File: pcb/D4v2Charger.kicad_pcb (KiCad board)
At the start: 2 copper layers, 21.6 x 20.6 mm, 16 parts, among them J1 Conn_01x02_Pin, U1 BQ25185DLHR

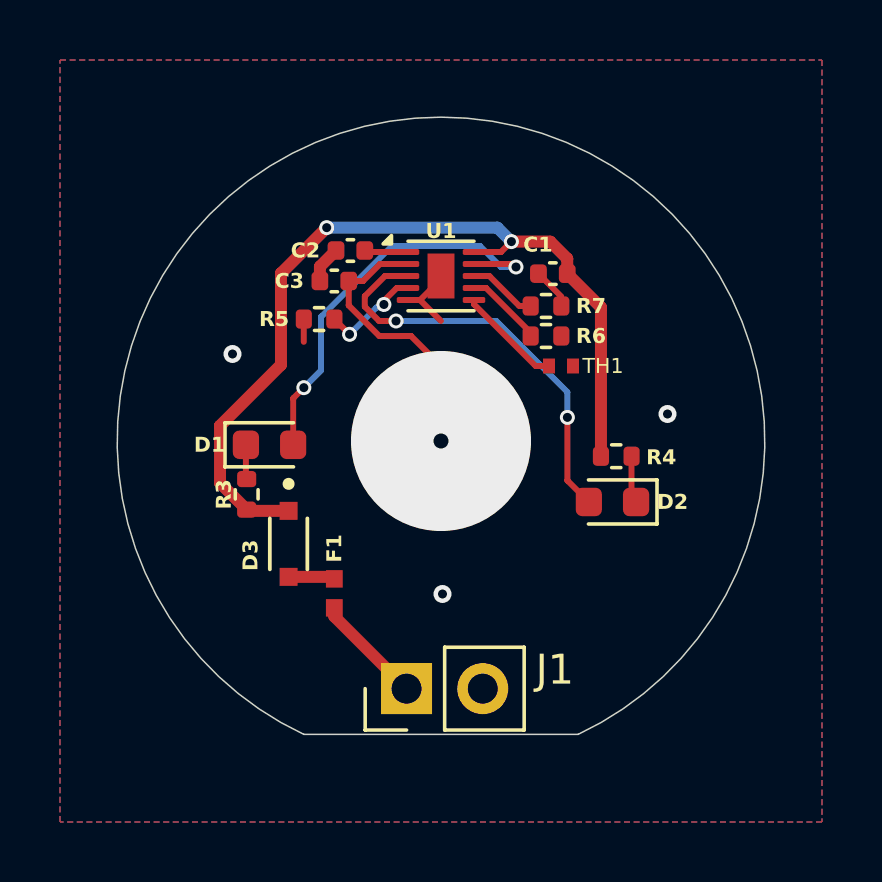
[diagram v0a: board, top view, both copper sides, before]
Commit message: update edge cuts
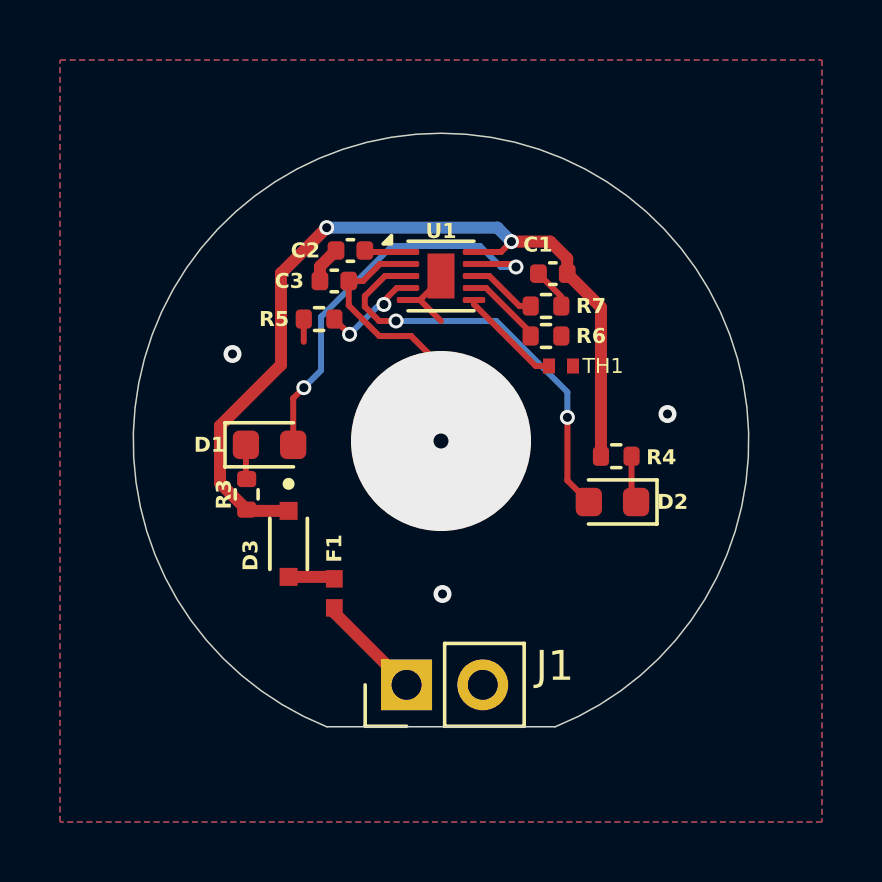
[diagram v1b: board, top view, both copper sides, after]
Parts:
- moved J1 0.13 mm to (170.3, 97.0)
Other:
- board size 21.6 x 20.6 mm -> 20.5 x 19.8 mm
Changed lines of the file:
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@@
 	(footprint "Connector_PinHeader_2.54mm:PinHeader_1x02_P2.54mm_Vertical"
 		(layer "F.Cu")
-		(at 170.302 97.155 90)
+		(at 170.302 97.028 90)
 		(descr "Through hole straight pin header, 1x02, 2.54mm pitch, single row")
 		(tags "Through hole pin header THT 1x02 2.54mm single row")
@@
 	)
 	(gr_arc
-		(start 166.878 98.679)
-		(mid 171.45 78.105)
-		(end 176.022 98.679)
+		(start 167.64 98.425)
+		(mid 171.45 78.641261)
+		(end 175.26 98.425)
 		(stroke
-			(width 4)
+			(width 2)
 			(type solid)
 		)
@@
 	)
 	(gr_arc
-		(start 166.878 98.679)
-		(mid 171.45 78.105)
-		(end 176.022 98.679)
+		(start 167.64 98.424998)
+		(mid 171.45 78.641259)
+		(end 175.26 98.424998)
 		(stroke
-			(width 4)
+			(width 2)
 			(type solid)
 		)
@@
 	)
 	(gr_arc
-		(start 166.878 98.679)
-		(mid 171.45 78.105)
-		(end 176.022 98.679)
+		(start 167.64 98.425)
+		(mid 171.45 78.641261)
+		(end 175.26 98.425)
 		(stroke
 			(width 0.05)
@@
 	)
 	(gr_line
-		(start 176.022 98.679)
-		(end 166.878 98.679)
+		(start 175.26 98.424998)
+		(end 167.640001 98.425)
 		(stroke
 			(width 0.05)
@@
 	)
 	(segment
+		(start 167.894 94.62)
+		(end 170.302 97.028)
+		(width 0.4)
+		(layer "F.Cu")
+		(net 14)
+	)
+	(segment
 		(start 167.894 94.463)
-		(end 167.894 94.747)
-		(width 0.4)
-		(layer "F.Cu")
-		(net 14)
-	)
-	(segment
-		(start 167.894 94.747)
-		(end 170.302 97.155)
-		(width 0.4)
-		(layer "F.Cu")
+		(end 167.894 94.62)
+		(width 0.4)
+		(layer "F.Cu")
